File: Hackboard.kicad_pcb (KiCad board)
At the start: 4 copper layers, 100 x 53.3 mm, 71 parts, among them J1 Conn_01x23_Socket, J2 Micro_SD_Card, J3 Conn_01x31_Socket, J4 Conn_01x08_Socket, J5 Conn_01x02_Pin, J6 USB_C_Receptacle_USB2.0_16P, J7 Barrel_Jack_Switch, Q1 NMOS, Q2 NMOS, Q3 NMOS, SW1 SW_SPST, U1 NCP164CSN330T1G, U2 AP63205WU, U3 STM32L476RGT6, U4 74LVC4245APW, U5 74LVC4245APW, U6 74LVC4245APW, U7 USBLC6-2SC6, U8 74LVC4245APW, U9 74LVC4245APW

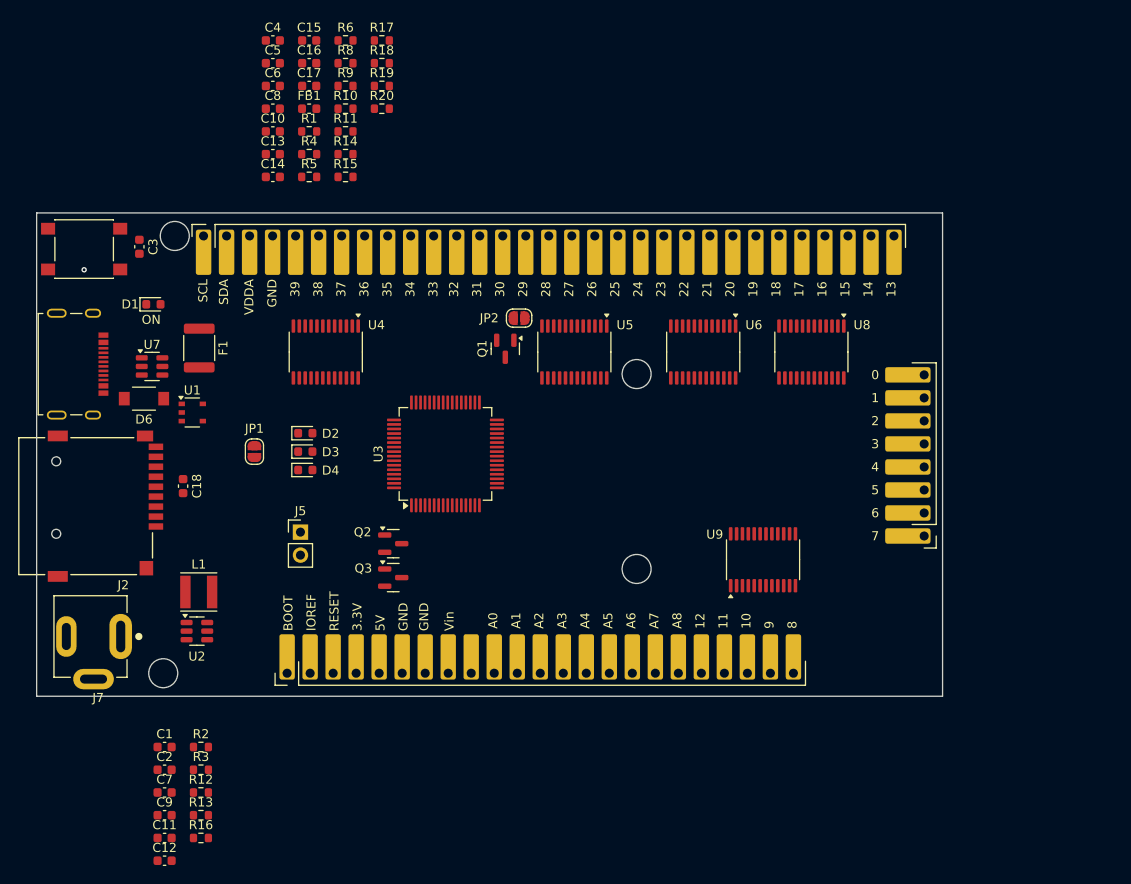
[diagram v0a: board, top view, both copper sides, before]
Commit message: Adjust pinout
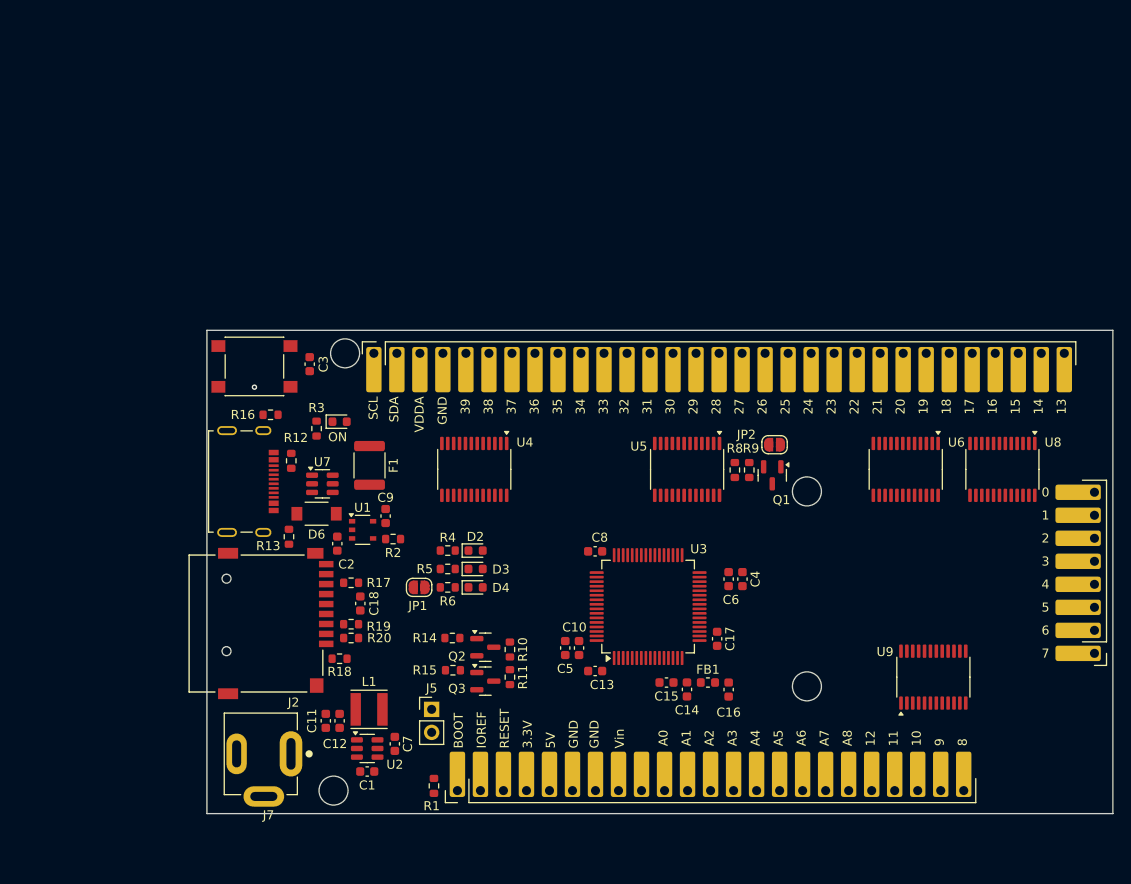
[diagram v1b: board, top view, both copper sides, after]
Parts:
- moved C16 83.2 mm to (159.3, 115.2), turned to 90 degrees
- moved C15 81.1 mm to (152.4, 114.4)
- moved C4 78.9 mm to (160.8, 103.0), turned to -90 degrees
- moved FB1 77.1 mm to (157.0, 114.4)
- moved C17 75.8 mm to (158.0, 109.6), turned to -90 degrees
- moved C6 74.1 mm to (159.3, 103.0), turned to -90 degrees
- moved R1 73.5 mm to (126.7, 125.8), turned to -90 degrees
- moved C14 72.7 mm to (154.7, 115.1), turned to 90 degrees
- moved C5 72.2 mm to (141.2, 110.6), turned to 90 degrees
- moved C13 67.2 mm to (144.5, 113.1), turned to 180 degrees
- moved C10 66.3 mm to (142.8, 110.6), turned to 90 degrees
- moved R18 65.9 mm to (116.3, 111.8), turned to 180 degrees
- moved R11 62.9 mm to (135.1, 113.8), turned to -90 degrees
- moved R10 62.4 mm to (135.1, 110.7), turned to -90 degrees
- moved R8 62.1 mm to (160.0, 90.9), turned to 90 degrees
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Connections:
- net CAN_RX_29_O renamed PWM_29_O
- net CAN_TX_30_O renamed PWM_30_O
- net GPIO_31_O renamed SD_SCK_31_O
- net PWM_25_O renamed CAN_TX_25_O
- net PWM_26_O renamed CAN_RX_26_O
- net SD_SCK_24_O renamed GPIO_24_O
- JP2 pad 1: PWM_28_O -> PWM_27_O
- Q2 pad 2: +3V3 -> VDDA
- Q3 pad 2: +3V3 -> VDDA
- R10 pad 2: +3V3 -> VDDA
- R11 pad 1: +3V3 -> VDDA
- U3 pad 2: GPIO_31 -> GPIO_24
- U3 pad 55: SD_SCK_24 -> SD_SCK_31
- U3 pad 56: PWM_25 -> PWM_30
- U3 pad 57: PWM_26 -> PWM_29
- U3 pad 58: PWM_27 -> PWM_28
- U3 pad 59: PWM_28 -> PWM_27
- U3 pad 61: CAN_RX_29 -> CAN_RX_26
- U3 pad 62: CAN_TX_30 -> CAN_TX_25
- U5 pad 12: GPIO_31 -> SD_SCK_31
- U5 pad 13: CAN_TX_30 -> PWM_30
- U5 pad 14: CAN_RX_29 -> PWM_29
- U5 pad 17: PWM_26 -> CAN_RX_26
- U5 pad 18: PWM_25 -> CAN_TX_25
- U5 pad 19: SD_SCK_24 -> GPIO_24
- U5 pad 6: PWM_27_O -> Net-(JP2-B)
- U5 pad 7: Net-(JP2-B) -> PWM_28_O
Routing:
- net SW_SWDIO: track 0.00 -> 82.3 mm
- net DAC_A0: track 82.3 -> 0.00 mm
- net VDDA: track 36.8 -> 0.00 mm
- net SCL: track 0.00 -> 36.8 mm
